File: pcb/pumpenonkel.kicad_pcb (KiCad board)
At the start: 2 copper layers, 105 x 157.5 mm, 21 parts, among them J1 Screw_Terminal_01x02, J10 NO_ON_JUMPER, J11 Screw_Terminal_01x02, J12 NO_ON_JUMPER, J13 Screw_Terminal_01x02, J14 Conn_01x02_Pin, J2 NO_ON_JUMPER, J3 Screw_Terminal_01x02, J4 NO_ON_JUMPER, J5 Screw_Terminal_01x02, J6 NO_ON_JUMPER, J7 Screw_Terminal_01x02, J8 NO_ON_JUMPER, J9 Screw_Terminal_01x02, K1 SANYOU_SRD_Form_C, K2 SANYOU_SRD_Form_C, K3 SANYOU_SRD_Form_C, K4 SANYOU_SRD_Form_C, K5 SANYOU_SRD_Form_C, K6 SANYOU_SRD_Form_C

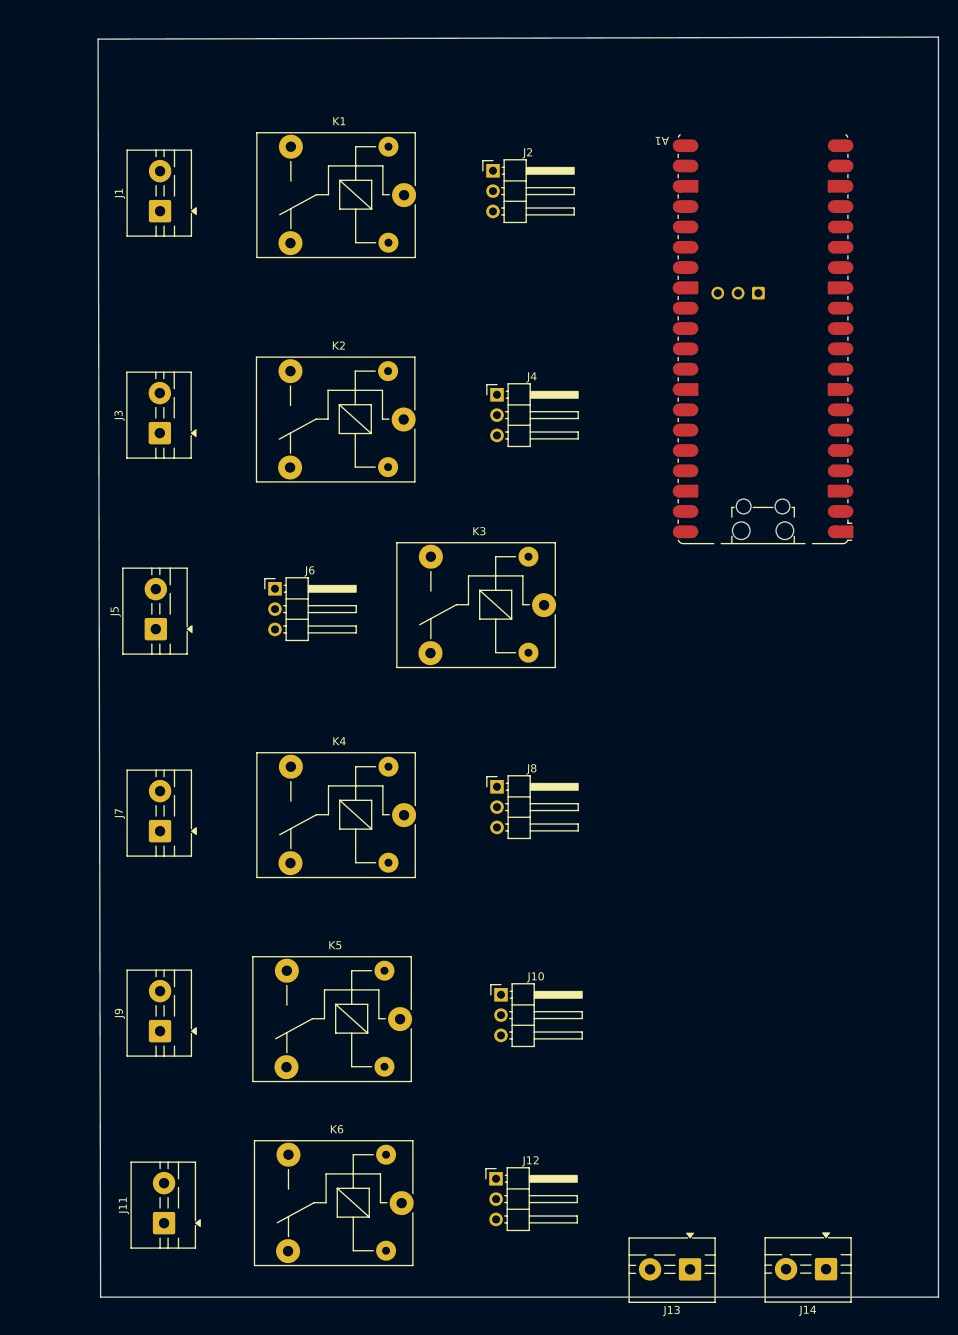
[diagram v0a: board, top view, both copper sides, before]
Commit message: Update PCB
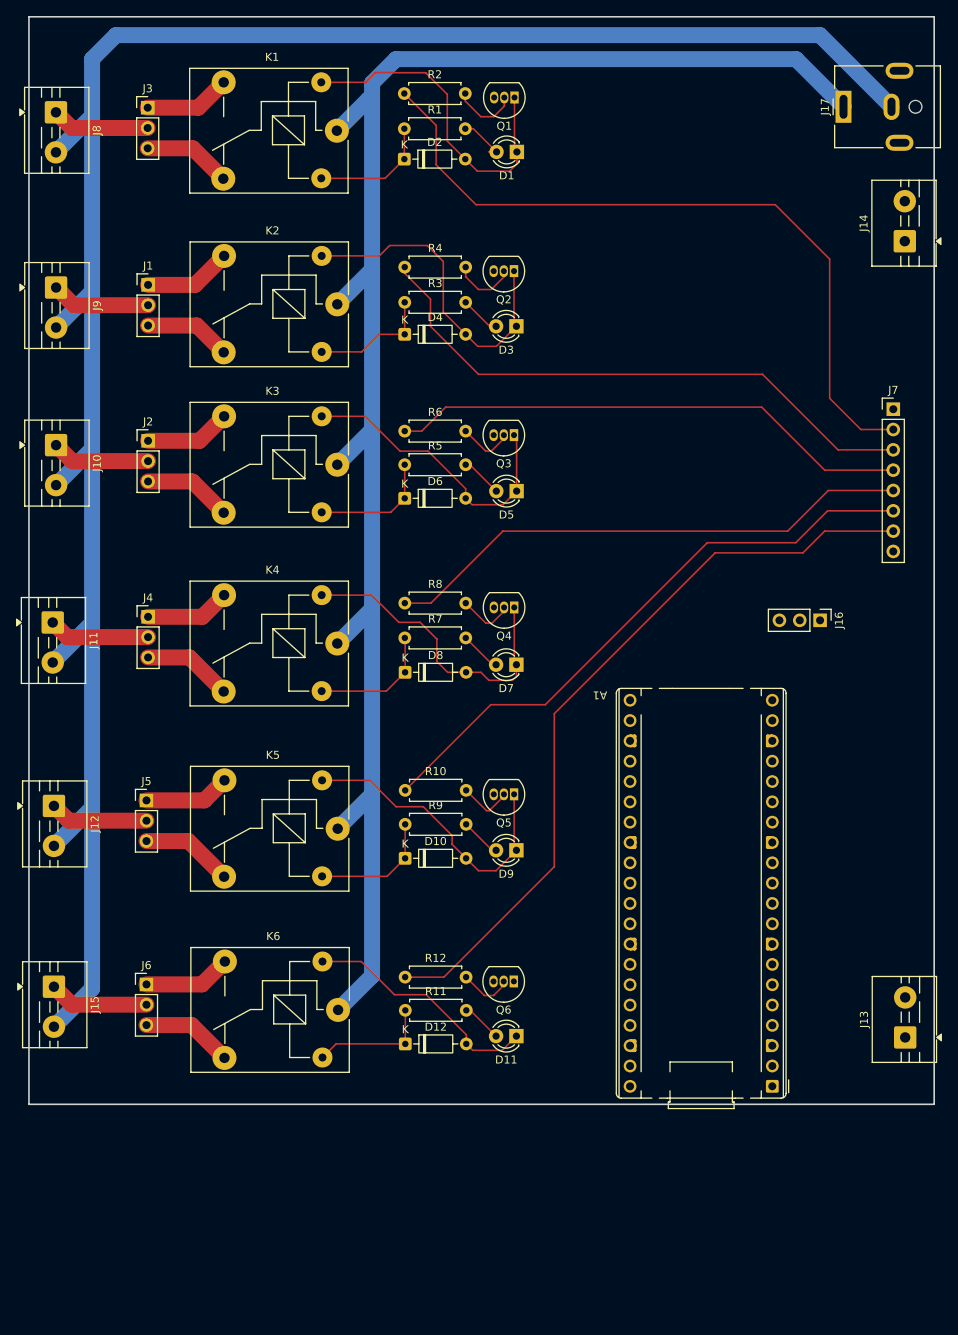
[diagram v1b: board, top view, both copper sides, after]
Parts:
- added D1: LED, LED_THT:LED_D3.0mm, F.Cu at (85.1, 44.6)
- added D10: 1N4148, Diode_THT:D_DO-35_SOD27_P7.62mm_Horizontal, F.Cu at (71.1, 132.9)
- added D11: LED, LED_THT:LED_D3.0mm, F.Cu at (85.0, 155.1)
- added D12: 1N4148, Diode_THT:D_DO-35_SOD27_P7.62mm_Horizontal, F.Cu at (71.2, 156.1)
- added D2: 1N4148, Diode_THT:D_DO-35_SOD27_P7.62mm_Horizontal, F.Cu at (71.0, 45.5)
- added D3: LED, LED_THT:LED_D3.0mm, F.Cu at (85.0, 66.4)
- added D4: 1N4148, Diode_THT:D_DO-35_SOD27_P7.62mm_Horizontal, F.Cu at (71.1, 67.4)
- added D5: LED, LED_THT:LED_D3.0mm, F.Cu at (85.1, 87.0)
- added D6: 1N4148, Diode_THT:D_DO-35_SOD27_P7.62mm_Horizontal, F.Cu at (71.1, 87.9)
- added D7: LED, LED_THT:LED_D3.0mm, F.Cu at (85.0, 108.7)
- added D8: 1N4148, Diode_THT:D_DO-35_SOD27_P7.62mm_Horizontal, F.Cu at (71.1, 109.7)
- added D9: LED, LED_THT:LED_D3.0mm, F.Cu at (85.0, 131.9)
- added J15: CHANNEL, TerminalBlock:TerminalBlock_MaiXu_MX126-5.0-02P_1x02_P5.00mm, F.Cu at (27.2, 148.9)
- added J16: Conn_01x03_Pin, Connector_PinHeader_2.54mm:PinHeader_1x03_P2.54mm_Vertical, F.Cu at (123.0, 103.2)
- added J17: Barrel_Jack, Connector_BarrelJack:BarrelJack_CUI_PJ-063AH_Horizontal, F.Cu at (125.9, 39.0)
- added Q1: BC337, Package_TO_SOT_THT:TO-92_Inline, F.Cu at (84.8, 37.8)
- added Q2: BC337, Package_TO_SOT_THT:TO-92_Inline, F.Cu at (84.7, 59.5)
- added Q3: BC337, Package_TO_SOT_THT:TO-92_Inline, F.Cu at (84.7, 80.0)
- added Q4: BC337, Package_TO_SOT_THT:TO-92_Inline, F.Cu at (84.8, 101.5)
- added Q5: BC337, Package_TO_SOT_THT:TO-92_Inline, F.Cu at (84.8, 124.9)
- added Q6: BC337, Package_TO_SOT_THT:TO-92_Inline, F.Cu at (84.7, 148.3)
- added R1: 1k, Resistor_THT:R_Axial_DIN0207_L6.3mm_D2.5mm_P7.62mm_Horizontal, F.Cu at (71.0, 41.7)
- added R10: 1k, Resistor_THT:R_Axial_DIN0207_L6.3mm_D2.5mm_P7.62mm_Horizontal, F.Cu at (71.1, 124.4)
- added R11: 1k, Resistor_THT:R_Axial_DIN0207_L6.3mm_D2.5mm_P7.62mm_Horizontal, F.Cu at (71.2, 151.9)
- added R12: 1k, Resistor_THT:R_Axial_DIN0207_L6.3mm_D2.5mm_P7.62mm_Horizontal, F.Cu at (71.1, 147.8)
- added R2: 1k, Resistor_THT:R_Axial_DIN0207_L6.3mm_D2.5mm_P7.62mm_Horizontal, F.Cu at (71.0, 37.3)
- added R3: 1k, Resistor_THT:R_Axial_DIN0207_L6.3mm_D2.5mm_P7.62mm_Horizontal, F.Cu at (71.1, 63.4)
- added R4: 1k, Resistor_THT:R_Axial_DIN0207_L6.3mm_D2.5mm_P7.62mm_Horizontal, F.Cu at (71.1, 59.0)
- added R5: 1k, Resistor_THT:R_Axial_DIN0207_L6.3mm_D2.5mm_P7.62mm_Horizontal, F.Cu at (71.1, 83.7)
- added R6: 1k, Resistor_THT:R_Axial_DIN0207_L6.3mm_D2.5mm_P7.62mm_Horizontal, F.Cu at (71.1, 79.5)
- added R7: 1k, Resistor_THT:R_Axial_DIN0207_L6.3mm_D2.5mm_P7.62mm_Horizontal, F.Cu at (71.1, 105.3)
- added R8: 1k, Resistor_THT:R_Axial_DIN0207_L6.3mm_D2.5mm_P7.62mm_Horizontal, F.Cu at (71.1, 101.0)
- added R9: 1k, Resistor_THT:R_Axial_DIN0207_L6.3mm_D2.5mm_P7.62mm_Horizontal, F.Cu at (71.1, 128.7)
- A1: footprint Module:RaspberryPi_Pico_W_SMD_HandSolder -> Module:RaspberryPi_Pico_Common_THT
- J1, J3, J5: value Screw_Terminal_01x02 -> Conn_01x03_Pin; footprint TerminalBlock:TerminalBlock_MaiXu_MX126-5.0-02P_1x02_P5.00mm -> Connector_PinHeader_2.54mm:PinHeader_1x03_P2.54mm_Vertical
- J10, J12, J8: value NO_ON_JUMPER -> CHANNEL; footprint Connector_PinHeader_2.54mm:PinHeader_1x03_P2.54mm_Horizontal -> TerminalBlock:TerminalBlock_MaiXu_MX126-5.0-02P_1x02_P5.00mm
- J11, J9: value Screw_Terminal_01x02 -> CHANNEL
- J14: value Conn_01x02_Pin -> Screw_Terminal_01x02
- J2, J4, J6: value NO_ON_JUMPER -> Conn_01x03_Pin; footprint Connector_PinHeader_2.54mm:PinHeader_1x03_P2.54mm_Horizontal -> Connector_PinHeader_2.54mm:PinHeader_1x03_P2.54mm_Vertical
- J7: value Screw_Terminal_01x02 -> Conn_01x08_Pin; footprint TerminalBlock:TerminalBlock_MaiXu_MX126-5.0-02P_1x02_P5.00mm -> Connector_PinHeader_2.54mm:PinHeader_1x08_P2.54mm_Vertical
- moved J14 128.9 mm to (133.6, 55.8), turned to 90 degrees
- moved J7 105.7 mm to (132.2, 76.8), turned to 0 degrees
- moved J8 100.7 mm to (27.5, 39.6), turned to -90 degrees
- moved J9 93.9 mm to (27.5, 61.5), turned to -90 degrees
- moved A1 93.5 mm to (117.0, 161.4)
- moved J10 88.4 mm to (27.5, 81.2), turned to -90 degrees
- moved J11 76.4 mm to (27.1, 103.4), turned to -90 degrees
- moved J12 72.3 mm to (27.2, 126.3), turned to -90 degrees
- moved J2 54.8 mm to (39.0, 80.7)
- moved J6 52.0 mm to (38.8, 148.7)
- moved J4 51.7 mm to (39.0, 102.7)
- moved J3 40.7 mm to (39.0, 39.1), turned to 0 degrees
- moved J13 39.5 mm to (133.6, 155.3), turned to 90 degrees
- moved K3 31.2 mm to (62.6, 83.7)
- moved K6 25.4 mm to (62.8, 151.8)
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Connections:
- A1 pad 1: D1 -> CH1
- A1 pad 13: DC_GND -> GND
- A1 pad 18: DC_GND -> GND
- A1 pad 2: D2 -> CH2
- A1 pad 23: DC_GND -> GND
- A1 pad 28: DC_GND -> GND
- A1 pad 3: DC_GND -> GND
- A1 pad 38: DC_GND -> GND
- A1 pad 39: +5V -> Net-(A1-VSYS)
- A1 pad 4: D3 -> CH3
- A1 pad 5: D4 -> CH4
- A1 pad 6: D5 -> CH5
- A1 pad 7: D6 -> CH6
- A1 pad 8: DC_GND -> GND
- J1 pad 2: AC_MINUS -> Net-(J1-Pin_2)
- J10 pad 2: Net-(J10-Pin_2) -> VAC
- J11 pad 2: AC_MINUS -> VAC
- J12 pad 2: Net-(J11-Pin_1) -> VAC
- J13 pad 1: AC_PLUS -> VAC
- J13 pad 2: AC_MINUS -> COM
- J14 pad 1: +5V -> VCC
- J14 pad 2: DC_GND -> GND
- J2 pad 2: Net-(J1-Pin_1) -> Net-(J10-Pin_1)
- J3 pad 2: AC_MINUS -> Net-(J3-Pin_2)
- J4 pad 2: Net-(J3-Pin_1) -> Net-(J11-Pin_1)
- J5 pad 2: AC_MINUS -> Net-(J12-Pin_1)
- J6 pad 2: Net-(J5-Pin_1) -> Net-(J15-Pin_1)
- J7 pad 1: Net-(J7-Pin_1) -> VCC
- J7 pad 2: AC_MINUS -> CH1
- J8 pad 1: Net-(J8-Pin_1) -> Net-(J3-Pin_2)
- J8 pad 2: Net-(J7-Pin_1) -> VAC
- J9 pad 1: Net-(J10-Pin_2) -> Net-(J1-Pin_2)
- J9 pad 2: AC_MINUS -> VAC
- K1 pad 1: AC_PLUS -> COM
- K1 pad 2: DC_GND -> Net-(D1-K)
- K1 pad 3: Net-(J2-Pin_1) -> Net-(J3-Pin_1)
- K1 pad 4: Net-(J2-Pin_3) -> Net-(J3-Pin_3)
- K1 pad 5: D1 -> VCC
- K2 pad 1: AC_PLUS -> COM
- K2 pad 2: DC_GND -> Net-(D3-K)
- K2 pad 3: Net-(J4-Pin_1) -> Net-(J1-Pin_1)
- K2 pad 4: Net-(J4-Pin_3) -> Net-(J1-Pin_3)
- K2 pad 5: D2 -> VCC
- K3 pad 1: AC_PLUS -> COM
- K3 pad 2: DC_GND -> Net-(D5-K)
- K3 pad 3: Net-(J6-Pin_1) -> Net-(J2-Pin_1)
- K3 pad 4: Net-(J6-Pin_3) -> Net-(J2-Pin_3)
- K3 pad 5: D3 -> VCC
- K4 pad 1: AC_PLUS -> COM
- K4 pad 2: DC_GND -> Net-(D7-K)
- K4 pad 3: Net-(J8-Pin_1) -> Net-(J4-Pin_1)
- K4 pad 4: Net-(J8-Pin_3) -> Net-(J4-Pin_3)
- K4 pad 5: D4 -> VCC
- K5 pad 1: AC_PLUS -> COM
- K5 pad 2: DC_GND -> Net-(D10-A)
- K5 pad 3: Net-(J10-Pin_1) -> Net-(J5-Pin_1)
- K5 pad 4: Net-(J10-Pin_3) -> Net-(J5-Pin_3)
- K5 pad 5: D5 -> VCC
- K6 pad 1: AC_PLUS -> COM
- K6 pad 2: DC_GND -> Net-(D11-K)
- K6 pad 3: Net-(J12-Pin_1) -> Net-(J6-Pin_1)
- K6 pad 4: Net-(J12-Pin_3) -> Net-(J6-Pin_3)
- K6 pad 5: D6 -> VCC
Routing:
- net VAC: track 0.00 -> 260.6 mm
- net COM: track 0.00 -> 210.8 mm
- net CH6: track 0.00 -> 95.3 mm
- net VCC: track 0.00 -> 92.3 mm
- net CH1: track 0.00 -> 91.6 mm
- net CH5: track 0.00 -> 75.5 mm
- net CH2: track 0.00 -> 73.0 mm
- net CH4: track 0.00 -> 66.9 mm
- net CH3: track 0.00 -> 65.6 mm
- net Net-(D1-K): track 0.00 -> 42.3 mm
- net Net-(D3-K): track 0.00 -> 41.8 mm
- net Net-(D7-K): track 0.00 -> 39.4 mm
- net Net-(D10-A): track 0.00 -> 37.8 mm
- net Net-(D5-K): track 0.00 -> 37.5 mm
- net Net-(D11-K): track 0.00 -> 30.2 mm
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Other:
- board size 105 x 157.5 mm -> 113.1 x 135.9 mm
